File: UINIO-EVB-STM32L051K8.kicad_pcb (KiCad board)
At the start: 2 copper layers, 34.4 x 36.6 mm, 28 parts, among them J1 Conn_01x14_Male, J2 Conn_01x14_Male, J3 Conn_01x04_Male, SW1 SW_Push, SW2 SW_Push, U1 ME6211C33M5G-N, U2 W25Q128JVSSIQ, U3 STM32L051K8U6, Y1 Crystal_GND24

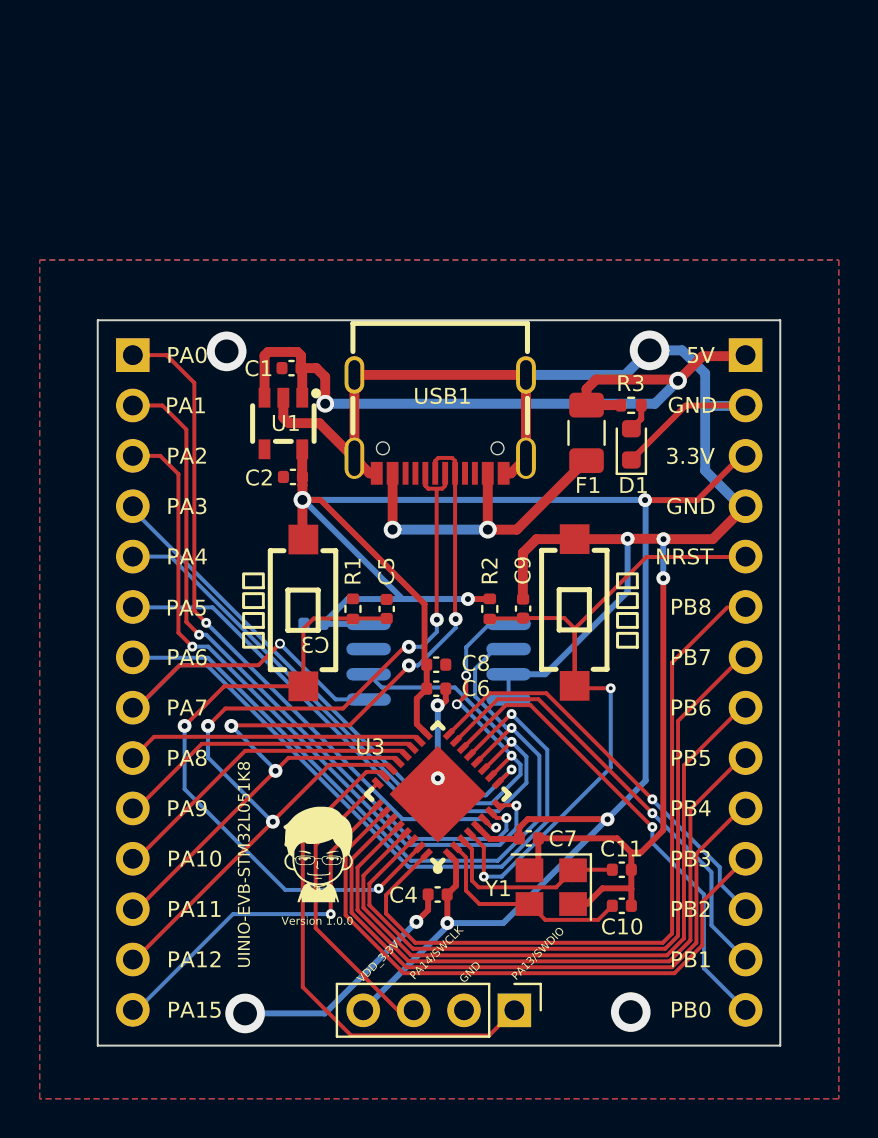
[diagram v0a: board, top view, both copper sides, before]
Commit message: Re-layout and wiring
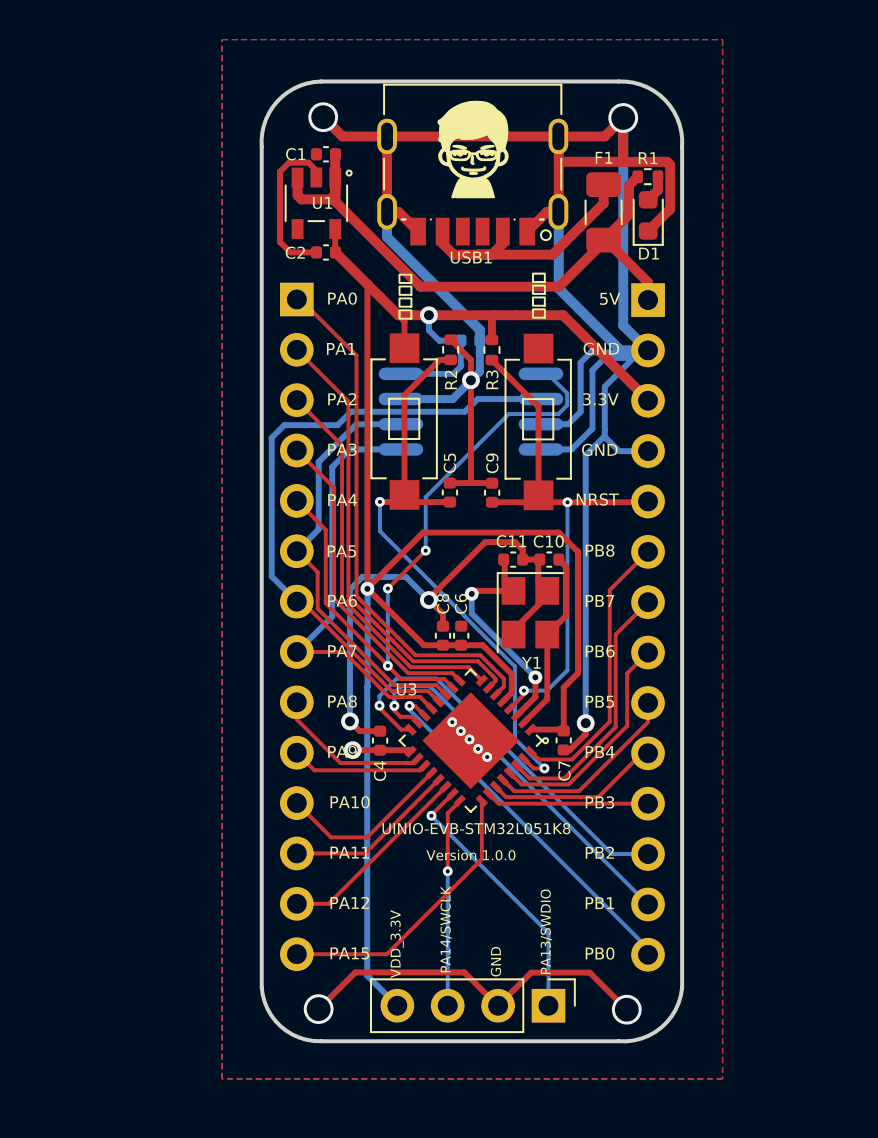
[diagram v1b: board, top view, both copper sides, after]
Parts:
- R1: value 10K -> 1K
- R2: value R -> 10K
- R3: value 1K -> R
- USB1: value USB_Type_C_16Pin -> USB_Type_C_6Pin; footprint Uinio:USB-C-SMD_TYPEC-304J-BCP16 -> Uinio:USB-TYPEC-250-BRP6L68
- moved ? 36.4 mm to (156.7, 86.0)
- moved R1 26.4 mm to (165.5, 87.5), turned to 180 degrees
- moved C10 17.8 mm to (160.5, 106.8), turned to 0 degrees
- moved C11 16.6 mm to (158.7, 106.8)
- moved C3 16.3 mm to (156.5, 95.8), turned to 180 degrees
- moved Y1 13.9 mm to (159.6, 109.5), turned to -90 degrees
- moved R2 13.2 mm to (155.5, 96.2)
- moved U2 12.7 mm to (156.6, 99.3)
- moved USB1 12.2 mm to (156.6, 87.9)
- moved D1 11.6 mm to (165.5, 89.5)
- moved C2 11.4 mm to (149.2, 91.3)
- moved U1 11.2 mm to (148.8, 88.8)
- moved F1 11.2 mm to (163.2, 89.3), turned to -90 degrees
- moved C1 10.9 mm to (149.2, 86.4)
- moved SW1 10.9 mm to (153.2, 99.8)
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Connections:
- J1 pad 12: /PA11/USB_Data_N -> /PA11
- J1 pad 13: /PA12/USB_Data_P -> /PA12
- R1 pad 1: GND -> Net-(D1-Pad2)
- R1 pad 2: /BOOT0 -> /VDD_5V
- R2 pad 1: /VDD_3.3V -> GND
- R2 pad 2: /NRST -> /BOOT0
- R3 pad 1: Net-(D1-Pad2) -> /VDD_3.3V
- R3 pad 2: /VDD_5V -> /NRST
- U3 pad 21: /PA11/USB_Data_N -> /PA11
- U3 pad 22: /PA12/USB_Data_P -> /PA12
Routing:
- net GND: track 124.1 -> 178.7 mm, vias 10 -> 13
- net /PA12/USB_Data_P: track 46.2 -> 0.00 mm, vias 4 -> 0
- net /PA11/USB_Data_N: track 43.4 -> 0.00 mm, vias 4 -> 0
- net /PA7/MOSI: track 50.4 -> 21.9 mm, vias 2 -> 0
- net /PB4: track 32.5 -> 8.50 mm
- net /PB5: track 33.8 -> 9.97 mm
- net /PB6: track 35.2 -> 11.5 mm
- net /PB7: track 36.5 -> 13.3 mm
- net /PB3: track 31.1 -> 8.23 mm
- net /PB8: track 36.7 -> 14.3 mm
- net /PA5/SCLK: track 37.7 -> 21.5 mm, vias 1 -> 0
- net /PA2: track 34.6 -> 19.7 mm, vias 2 -> 0
- net /PA1: track 35.3 -> 23.2 mm, vias 2 -> 0
- net /PA13/SWDIO: track 25.4 -> 13.6 mm, vias 0 -> 1
- net /NRST: track 37.2 -> 27.2 mm
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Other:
- board size 34.4 x 36.6 mm -> 21.2 x 48.4 mm
